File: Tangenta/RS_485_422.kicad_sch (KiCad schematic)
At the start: 32 parts, among them J10 Conn_01x02_Pin, Q3 BSS138, U16 ADM2582E, U17 TPCDSOT23-SM712, U18 TPCDSOT23-SM712

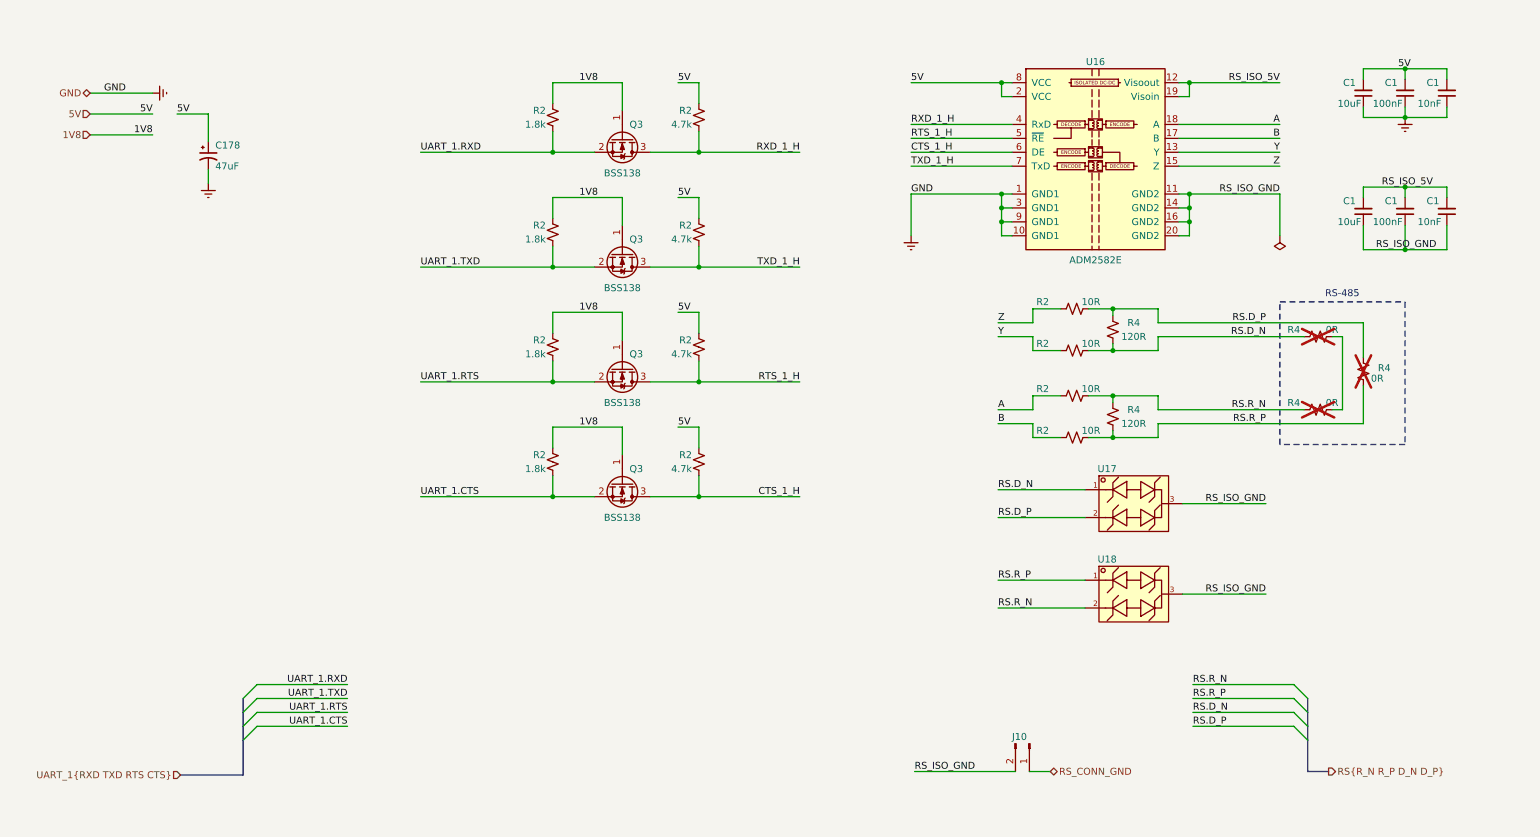
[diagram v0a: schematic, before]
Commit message: initialize branch
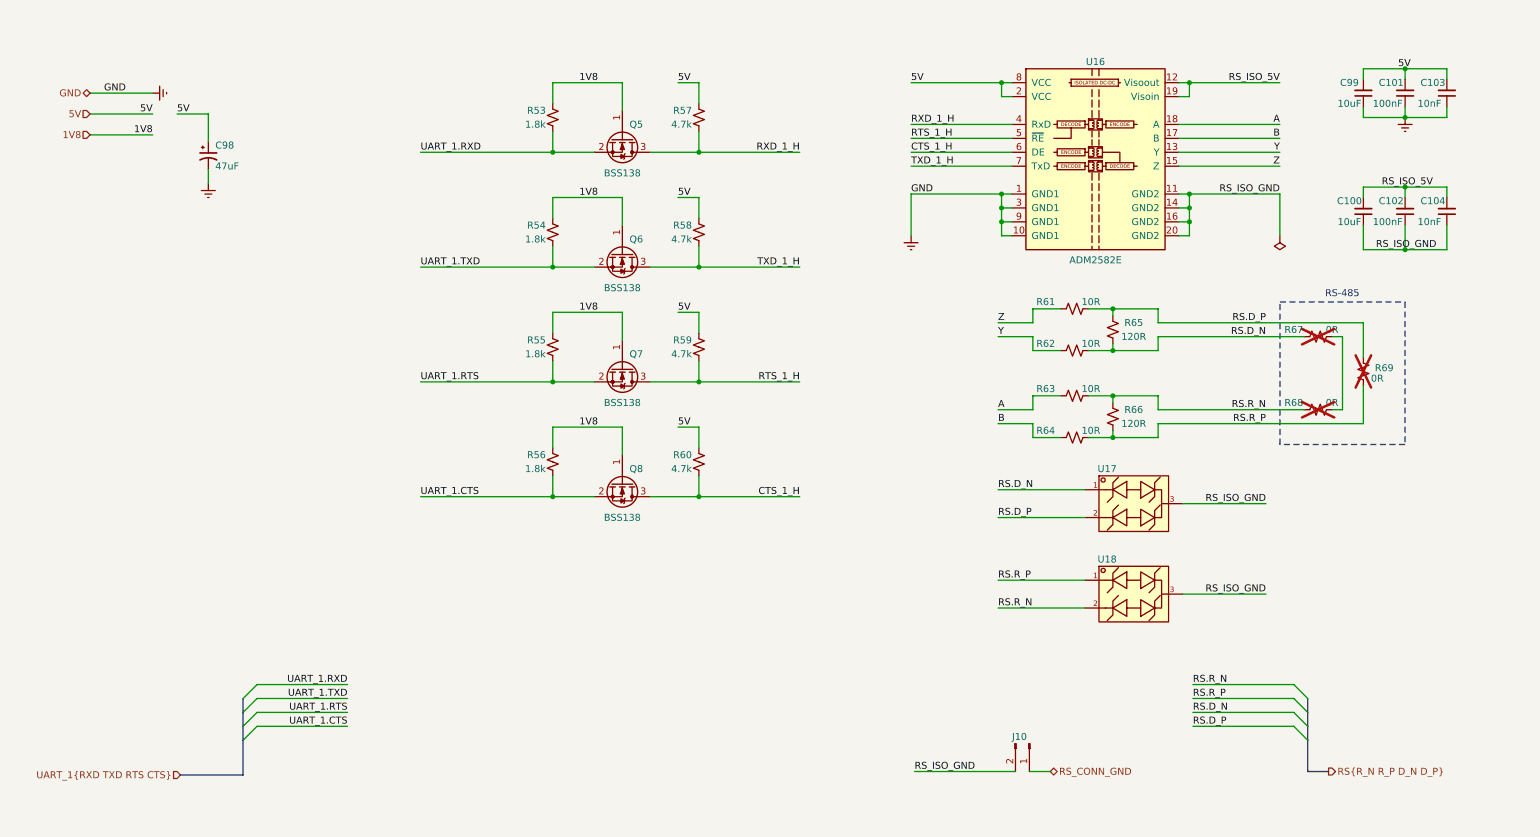
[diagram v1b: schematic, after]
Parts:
- renumbered C1 to C100, C1 to C101, C1 to C102, C1 to C103, C1 to C104, C178 to C98, C1 to C99, Q3 to Q5, Q3 to Q6, Q3 to Q7, Q3 to Q8, R2 to R53, R2 to R54, R2 to R55, R2 to R56, R2 to R57, R2 to R58, R2 to R59, R2 to R60, R2 to R61, R2 to R62, R2 to R63, R2 to R64, R4 to R65, R4 to R66, R4 to R67, R4 to R68, R4 to R69

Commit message: ESD_RS485, SOIC-20W_7.5x12.8mm_P1
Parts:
- U17, U18: footprint ESD_RS485:ESD_RS485 -> CholaFootprintsPrjLib:ESD_RS485
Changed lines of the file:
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@@
       (effects (font (size 1.27 1.27)) hide)
     )
-    (property "Footprint" "ESD_RS485:ESD_RS485" (at 218.821 142.621 0)
+    (property "Footprint" "CholaFootprintsPrjLib:ESD_RS485" (at 218.821 142.621 0)
       (effects (font (size 1.27 1.27) italic) hide)
     )
@@
     )
   )
-  (symbol (lib_id "CholaSymbolsPrjLib:TPCDSOT23-SM712") (at 216.916 111.125 0) (unit 1)
+  (symbol (lib_name "TPCDSOT23-SM712_1") (lib_id "CholaSymbolsPrjLib:TPCDSOT23-SM712") (at 216.916 111.125 0) (unit 1)
     (in_bom yes) (on_board yes) (dnp no)
     (property "Reference" "U17" (at 210.566 104.775 0)
@@
       (effects (font (size 1.27 1.27)) (justify left) hide)
     )
-    (property "Footprint" "ESD_RS485:ESD_RS485" (at 218.821 126.111 0)
+    (property "Footprint" "CholaFootprintsPrjLib:ESD_RS485" (at 218.821 126.111 0)
       (effects (font (size 1.27 1.27) italic) hide)
     )

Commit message: CAP_L5, CR2032_HOL, Ferrite_Bead, XTAL_24-25
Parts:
- C98: footprint CAP_L5:CAP_L5 -> CholaFootprintsPrjLib:CAP_L5
- U16: footprint Package_SO:SOIC-20W_7.5x12.8mm_P1.27mm -> CholaFootprintsPrjLib:SOIC-20W_7.5x12.8mm_P1.27mm
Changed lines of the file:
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@@
       (effects (font (size 1.27 1.27)) (justify left))
     )
-    (property "Footprint" "CAP_L5:CAP_L5" (at 46.99 65.405 0)
+    (property "Footprint" "CholaFootprintsPrjLib:CAP_L5" (at 46.99 65.405 0)
       (effects (font (size 1.27 1.27) italic) hide)
     )
@@
       (effects (font (size 1.27 1.27)))
     )
-    (property "Footprint" "Package_SO:SOIC-20W_7.5x12.8mm_P1.27mm" (at 210.185 67.31 0)
-      (effects (font (size 1.27 1.27)) hide)
-    )
+    (property "Footprint" "CholaFootprintsPrjLib:SOIC-20W_7.5x12.8mm_P1.27mm" (at 210.185 67.31 0)
+      (effects (font (size 1.27 1.27)) hide)
+    )

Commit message: Removing component association with previous project (local) libraries.
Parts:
- C100, C101, C102, C103, C104, C99: symbol CholaSymbolsPrjLib:C_Small -> C_Small:C_Small
- C98: footprint CholaFootprintsPrjLib:CAP_L5 -> CAP_L5:CAP_L5; symbol CholaSymbolsPrjLib:16CE47FSS -> 16CE47FSS:16CE47FSS
- J10: symbol CholaSymbolsPrjLib:Conn_01x02_Pin -> Conn_01x02_Pin:Conn_01x02_Pin
- Q5, Q6, Q7, Q8: symbol CholaSymbolsPrjLib:BSS138 -> BSS138:BSS138
- R53, R54, R55, R56, R57, R58, R59, R60, R61, R62, R63, R64, R65, R66, R67, R68, R69: symbol CholaSymbolsPrjLib:R_Small_US -> R_Small_US:R_Small_US
- U16: footprint CholaFootprintsPrjLib:SOIC-20W_7.5x12.8mm_P1.27mm -> SOIC-20W_7.5x12.8mm_P1.27mm:SOIC-20W_7.5x12.8mm_P1.27mm; symbol CholaSymbolsPrjLib:ADM2582E -> ADM2582E:ADM2582E
- U17, U18: footprint CholaFootprintsPrjLib:ESD_RS485 -> ESD_RS485:ESD_RS485; symbol CholaSymbolsPrjLib:TPCDSOT23-SM712 -> TPCDSOT23-SM712:TPCDSOT23-SM712
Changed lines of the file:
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@@
 	)
 	(symbol
-		(lib_id "CholaSymbolsPrjLib:R_Small_US")
+		(lib_id "R_Small_US:R_Small_US")
 		(at 137.795 40.64 180)
 		(unit 1)
@@
 	)
 	(symbol
-		(lib_id "CholaSymbolsPrjLib:R_Small_US")
+		(lib_id "R_Small_US:R_Small_US")
 		(at 206.375 75.565 270)
 		(unit 1)
@@
 	)
 	(symbol
-		(lib_id "CholaSymbolsPrjLib:R_Small_US")
+		(lib_id "R_Small_US:R_Small_US")
 		(at 250.825 80.645 270)
 		(unit 1)
@@
 	)
 	(symbol
-		(lib_id "CholaSymbolsPrjLib:R_Small_US")
+		(lib_id "R_Small_US:R_Small_US")
 		(at 137.795 82.55 180)
 		(unit 1)
@@
 	)
 	(symbol
-		(lib_id "CholaSymbolsPrjLib:R_Small_US")
+		(lib_id "R_Small_US:R_Small_US")
 		(at 206.375 91.44 270)
 		(unit 1)
@@
 	)
 	(symbol
-		(lib_id "CholaSymbolsPrjLib:R_Small_US")
+		(lib_id "R_Small_US:R_Small_US")
 		(at 213.36 79.375 0)
 		(unit 1)
@@
 	)
 	(symbol
-		(lib_id "CholaSymbolsPrjLib:C_Small")
+		(lib_id "C_Small:C_Small")
 		(at 266.7 36.195 180)
 		(unit 1)
@@
 	)
 	(symbol
-		(lib_id "CholaSymbolsPrjLib:BSS138")
+		(lib_id "BSS138:BSS138")
 		(at 123.825 65.405 270)
 		(unit 1)
@@
 	)
 	(symbol
-		(lib_id "CholaSymbolsPrjLib:R_Small_US")
+		(lib_id "R_Small_US:R_Small_US")
 		(at 206.375 99.06 270)
 		(unit 1)
@@
 	)
 	(symbol
-		(lib_id "CholaSymbolsPrjLib:R_Small_US")
+		(lib_id "R_Small_US:R_Small_US")
 		(at 259.08 86.995 0)
 		(unit 1)
@@
 	)
 	(symbol
-		(lib_id "CholaSymbolsPrjLib:C_Small")
+		(lib_id "C_Small:C_Small")
 		(at 266.7 57.785 180)
 		(unit 1)
@@
 	)
 	(symbol
-		(lib_id "CholaSymbolsPrjLib:R_Small_US")
+		(lib_id "R_Small_US:R_Small_US")
 		(at 206.375 83.185 270)
 		(unit 1)
@@
 	)
 	(symbol
-		(lib_id "CholaSymbolsPrjLib:C_Small")
+		(lib_id "C_Small:C_Small")
 		(at 259.08 36.195 180)
 		(unit 1)
@@
 	)
 	(symbol
-		(lib_id "CholaSymbolsPrjLib:R_Small_US")
+		(lib_id "R_Small_US:R_Small_US")
 		(at 137.795 61.595 180)
 		(unit 1)
@@
 	)
 	(symbol
-		(lib_id "CholaSymbolsPrjLib:BSS138")
+		(lib_id "BSS138:BSS138")
 		(at 123.825 44.45 270)
 		(unit 1)
@@
 	)
 	(symbol
-		(lib_id "CholaSymbolsPrjLib:16CE47FSS")
+		(lib_id "16CE47FSS:16CE47FSS")
 		(at 48.26 47.625 0)
 		(unit 1)
@@
 			)
 		)
-		(property "Footprint" "CholaFootprintsPrjLib:CAP_L5"
+		(property "Footprint" "CAP_L5:CAP_L5"
 			(at 46.99 65.405 0)
 			(effects
@@
 	)
 	(symbol
-		(lib_id "CholaSymbolsPrjLib:R_Small_US")
+		(lib_id "R_Small_US:R_Small_US")
 		(at 111.125 82.55 180)
 		(unit 1)
@@
 	)
 	(symbol
-		(lib_id "CholaSymbolsPrjLib:R_Small_US")
+		(lib_id "R_Small_US:R_Small_US")
 		(at 111.125 103.505 180)
 		(unit 1)
@@
 	)
 	(symbol
-		(lib_id "CholaSymbolsPrjLib:TPCDSOT23-SM712")
+		(lib_id "TPCDSOT23-SM712:TPCDSOT23-SM712")
 		(at 216.916 127.635 0)
 		(unit 1)
@@
 			)
 		)
-		(property "Footprint" "CholaFootprintsPrjLib:ESD_RS485"
+		(property "Footprint" "ESD_RS485:ESD_RS485"
 			(at 218.821 142.621 0)
 			(effects
@@
 	)
 	(symbol
-		(lib_id "CholaSymbolsPrjLib:R_Small_US")
+		(lib_id "R_Small_US:R_Small_US")
 		(at 111.125 40.64 180)
 		(unit 1)
@@
 	)
 	(symbol
-		(lib_id "CholaSymbolsPrjLib:C_Small")
+		(lib_id "C_Small:C_Small")
 		(at 274.32 57.785 180)
 		(unit 1)
@@
 	)
 	(symbol
-		(lib_id "CholaSymbolsPrjLib:BSS138")
+		(lib_id "BSS138:BSS138")
 		(at 123.825 86.36 270)
 		(unit 1)
@@
 	)
 	(symbol
-		(lib_id "CholaSymbolsPrjLib:ADM2582E")
+		(lib_id "ADM2582E:ADM2582E")
 		(at 210.185 49.53 0)
 		(unit 1)
@@
 			)
 		)
-		(property "Footprint" "CholaFootprintsPrjLib:SOIC-20W_7.5x12.8mm_P1.27mm"
+		(property "Footprint" "SOIC-20W_7.5x12.8mm_P1.27mm:SOIC-20W_7.5x12.8mm_P1.27mm"
 			(at 210.185 67.31 0)
 			(effects
@@
 	)
 	(symbol
-		(lib_id "CholaSymbolsPrjLib:R_Small_US")
+		(lib_id "R_Small_US:R_Small_US")
 		(at 137.795 103.505 180)
 		(unit 1)
@@
 	)
 	(symbol
-		(lib_id "CholaSymbolsPrjLib:BSS138")
+		(lib_id "BSS138:BSS138")
 		(at 123.825 107.315 270)
 		(unit 1)
@@
 	)
 	(symbol
-		(lib_id "CholaSymbolsPrjLib:C_Small")
+		(lib_id "C_Small:C_Small")
 		(at 274.32 36.195 180)
 		(unit 1)
@@
 	)
 	(symbol
-		(lib_id "CholaSymbolsPrjLib:R_Small_US")
+		(lib_id "R_Small_US:R_Small_US")
 		(at 111.125 61.595 180)
 		(unit 1)
@@
 	)
 	(symbol
-		(lib_id "CholaSymbolsPrjLib:R_Small_US")
+		(lib_id "R_Small_US:R_Small_US")
 		(at 250.825 93.98 270)
 		(unit 1)
@@
 	)
 	(symbol
-		(lib_id "CholaSymbolsPrjLib:Conn_01x02_Pin")
+		(lib_id "Conn_01x02_Pin:Conn_01x02_Pin")
 		(at 198.12 154.94 270)
 		(unit 1)
@@
 	)
 	(symbol
-		(lib_id "CholaSymbolsPrjLib:R_Small_US")
+		(lib_id "R_Small_US:R_Small_US")
 		(at 213.36 95.25 180)
 		(unit 1)
@@
 	(symbol
 		(lib_name "TPCDSOT23-SM712_1")
-		(lib_id "CholaSymbolsPrjLib:TPCDSOT23-SM712")
+		(lib_id "TPCDSOT23-SM712:TPCDSOT23-SM712")
 		(at 216.916 111.125 0)
 		(unit 1)
@@
 			)
 		)
-		(property "Footprint" "CholaFootprintsPrjLib:ESD_RS485"
+		(property "Footprint" "ESD_RS485:ESD_RS485"
 			(at 218.821 126.111 0)
 			(effects
@@
 	)
 	(symbol
-		(lib_id "CholaSymbolsPrjLib:C_Small")
+		(lib_id "C_Small:C_Small")
 		(at 259.08 57.785 180)
 		(unit 1)

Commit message: Fixes, continued...
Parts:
- C100, C101, C102, C103, C104, C99: symbol C_Small:C_Small -> Device:C_Small
- J10: symbol Conn_01x02_Pin:Conn_01x02_Pin -> Connector_Generic:Conn_01x02_Pin
- Q5, Q6, Q7, Q8: symbol BSS138:BSS138 -> Transistor_FET:BSS138
- R53, R54, R55, R56, R57, R58, R59, R60, R61, R62, R63, R64, R65, R66, R67, R68, R69: symbol R_Small_US:R_Small_US -> Device:R_Small_US
- U16: symbol ADM2582E:ADM2582E -> ADM2582EBRWZ:ADM2582EBRWZ-REEL7
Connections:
- net 1V8: no longer Q5.1 (G), Q6.1 (G), Q7.1 (G), Q8.1 (G), R53.2, R54.2, R55.2, R56.2
- net 5V: no longer C101.2, C103.2, C99.2, R57.2, R58.2, R59.2, R60.2, U16.2 (VCC), U16.8 (VCC)
- net A: no longer R63.2, U16.18 (A)
- net B: no longer R64.2, U16.17 (B)
- net CTS_1_H: no longer Q8.3 (D), R60.1, U16.6 (DE)
- net GNDREF: no longer C101.1, C103.1, C99.1, U16.1 (GND1), U16.10 (GND1), U16.3 (GND1), U16.9 (GND1)
- net RS.D_N: no longer R62.1, R65.2, R67.2
- net RS.D_P: no longer R61.1, R65.1, R69.1
- net RS.R_N: no longer R63.1, R66.2, R68.2
- net RS.R_P: no longer R64.1, R66.1, R69.2
- net RS_CONN_GND: no longer J10.1 (Pin_1)
- net RS_ISO_5V: no longer C100.2, C102.2, C104.2, U16.12 (Visoout), U16.19 (Visoin)
- net RS_ISO_GND: no longer C100.1, C102.1, C104.1, J10.2 (Pin_2), U16.11 (GND2), U16.14 (GND2), U16.16 (GND2), U16.20 (GND2)
- net RTS_1_H: no longer Q7.3 (D), R59.1, U16.5 (~{RE})
- net RXD_1_H: no longer Q5.3 (D), R57.1, U16.4 (RxD)
- net TXD_1_H: no longer Q6.3 (D), R58.1, U16.7 (TxD)
- net UART_1.CTS: no longer Q8.2 (S), R56.1
- net UART_1.RTS: no longer Q7.2 (S), R55.1
- net UART_1.RXD: no longer Q5.2 (S), R53.1
- net UART_1.TXD: no longer Q6.2 (S), R54.1
- net Y: no longer R62.2, U16.13 (Y)
- net Z: no longer R61.2, U16.15 (Z)
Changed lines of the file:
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@@
 	)
 	(symbol
-		(lib_id "R_Small_US:R_Small_US")
+		(lib_id "Device:R_Small_US")
 		(at 137.795 40.64 180)
 		(unit 1)
@@
 	)
 	(symbol
-		(lib_id "R_Small_US:R_Small_US")
+		(lib_id "Device:R_Small_US")
 		(at 206.375 75.565 270)
 		(unit 1)
@@
 	)
 	(symbol
-		(lib_id "R_Small_US:R_Small_US")
+		(lib_id "Device:R_Small_US")
 		(at 250.825 80.645 270)
 		(unit 1)
@@
 	)
 	(symbol
-		(lib_id "R_Small_US:R_Small_US")
+		(lib_id "Device:R_Small_US")
 		(at 137.795 82.55 180)
 		(unit 1)
@@
 	)
 	(symbol
-		(lib_id "R_Small_US:R_Small_US")
+		(lib_id "Device:R_Small_US")
 		(at 206.375 91.44 270)
 		(unit 1)
@@
 	)
 	(symbol
-		(lib_id "R_Small_US:R_Small_US")
+		(lib_id "Device:R_Small_US")
 		(at 213.36 79.375 0)
 		(unit 1)
@@
 	)
 	(symbol
-		(lib_id "C_Small:C_Small")
+		(lib_id "Device:C_Small")
 		(at 266.7 36.195 180)
 		(unit 1)
@@
 	)
 	(symbol
-		(lib_id "BSS138:BSS138")
+		(lib_id "Transistor_FET:BSS138")
 		(at 123.825 65.405 270)
 		(unit 1)
@@
 	)
 	(symbol
-		(lib_id "R_Small_US:R_Small_US")
+		(lib_id "Device:R_Small_US")
 		(at 206.375 99.06 270)
 		(unit 1)
@@
 	)
 	(symbol
-		(lib_id "R_Small_US:R_Small_US")
+		(lib_id "Device:R_Small_US")
 		(at 259.08 86.995 0)
 		(unit 1)
@@
 	)
 	(symbol
-		(lib_id "C_Small:C_Small")
+		(lib_id "Device:C_Small")
 		(at 266.7 57.785 180)
 		(unit 1)
@@
 	)
 	(symbol
-		(lib_id "R_Small_US:R_Small_US")
+		(lib_id "Device:R_Small_US")
 		(at 206.375 83.185 270)
 		(unit 1)
@@
 	)
 	(symbol
-		(lib_id "C_Small:C_Small")
+		(lib_id "Device:C_Small")
 		(at 259.08 36.195 180)
 		(unit 1)
@@
 	)
 	(symbol
-		(lib_id "R_Small_US:R_Small_US")
+		(lib_id "Device:R_Small_US")
 		(at 137.795 61.595 180)
 		(unit 1)
@@
 	)
 	(symbol
-		(lib_id "BSS138:BSS138")
+		(lib_id "Transistor_FET:BSS138")
 		(at 123.825 44.45 270)
 		(unit 1)
@@
 	)
 	(symbol
-		(lib_id "R_Small_US:R_Small_US")
+		(lib_id "Device:R_Small_US")
 		(at 111.125 82.55 180)
 		(unit 1)
@@
 	)
 	(symbol
-		(lib_id "R_Small_US:R_Small_US")
+		(lib_id "Device:R_Small_US")
 		(at 111.125 103.505 180)
 		(unit 1)
@@
 	)
 	(symbol
-		(lib_id "R_Small_US:R_Small_US")
+		(lib_id "Device:R_Small_US")
 		(at 111.125 40.64 180)
 		(unit 1)
@@
 	)
 	(symbol
-		(lib_id "C_Small:C_Small")
+		(lib_id "Device:C_Small")
 		(at 274.32 57.785 180)
 		(unit 1)
@@
 	)
 	(symbol
-		(lib_id "BSS138:BSS138")
+		(lib_id "Transistor_FET:BSS138")
 		(at 123.825 86.36 270)
 		(unit 1)
@@
 	)
 	(symbol
-		(lib_id "ADM2582E:ADM2582E")
+		(lib_id "ADM2582EBRWZ:ADM2582EBRWZ-REEL7")
 		(at 210.185 49.53 0)
 		(unit 1)
@@
 	)
 	(symbol
-		(lib_id "R_Small_US:R_Small_US")
+		(lib_id "Device:R_Small_US")
 		(at 137.795 103.505 180)
 		(unit 1)
@@
 	)
 	(symbol
-		(lib_id "BSS138:BSS138")
+		(lib_id "Transistor_FET:BSS138")
 		(at 123.825 107.315 270)
 		(unit 1)
@@
 	)
 	(symbol
-		(lib_id "C_Small:C_Small")
+		(lib_id "Device:C_Small")
 		(at 274.32 36.195 180)
 		(unit 1)
@@
 	)
 	(symbol
-		(lib_id "R_Small_US:R_Small_US")
+		(lib_id "Device:R_Small_US")
 		(at 111.125 61.595 180)
 		(unit 1)
@@
 	)
 	(symbol
-		(lib_id "R_Small_US:R_Small_US")
+		(lib_id "Device:R_Small_US")
 		(at 250.825 93.98 270)
 		(unit 1)
@@
 	)
 	(symbol
-		(lib_id "Conn_01x02_Pin:Conn_01x02_Pin")
+		(lib_id "Connector_Generic:Conn_01x02_Pin")
 		(at 198.12 154.94 270)
 		(unit 1)
@@
 	)
 	(symbol
-		(lib_id "R_Small_US:R_Small_US")
+		(lib_id "Device:R_Small_US")
 		(at 213.36 95.25 180)
 		(unit 1)
@@
 	)
 	(symbol
-		(lib_id "C_Small:C_Small")
+		(lib_id "Device:C_Small")
 		(at 259.08 57.785 180)
 		(unit 1)
